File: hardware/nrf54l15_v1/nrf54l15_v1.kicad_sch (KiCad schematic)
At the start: 2 parts, among them U1 MAXM86161EFD+, U2 VL53L0X

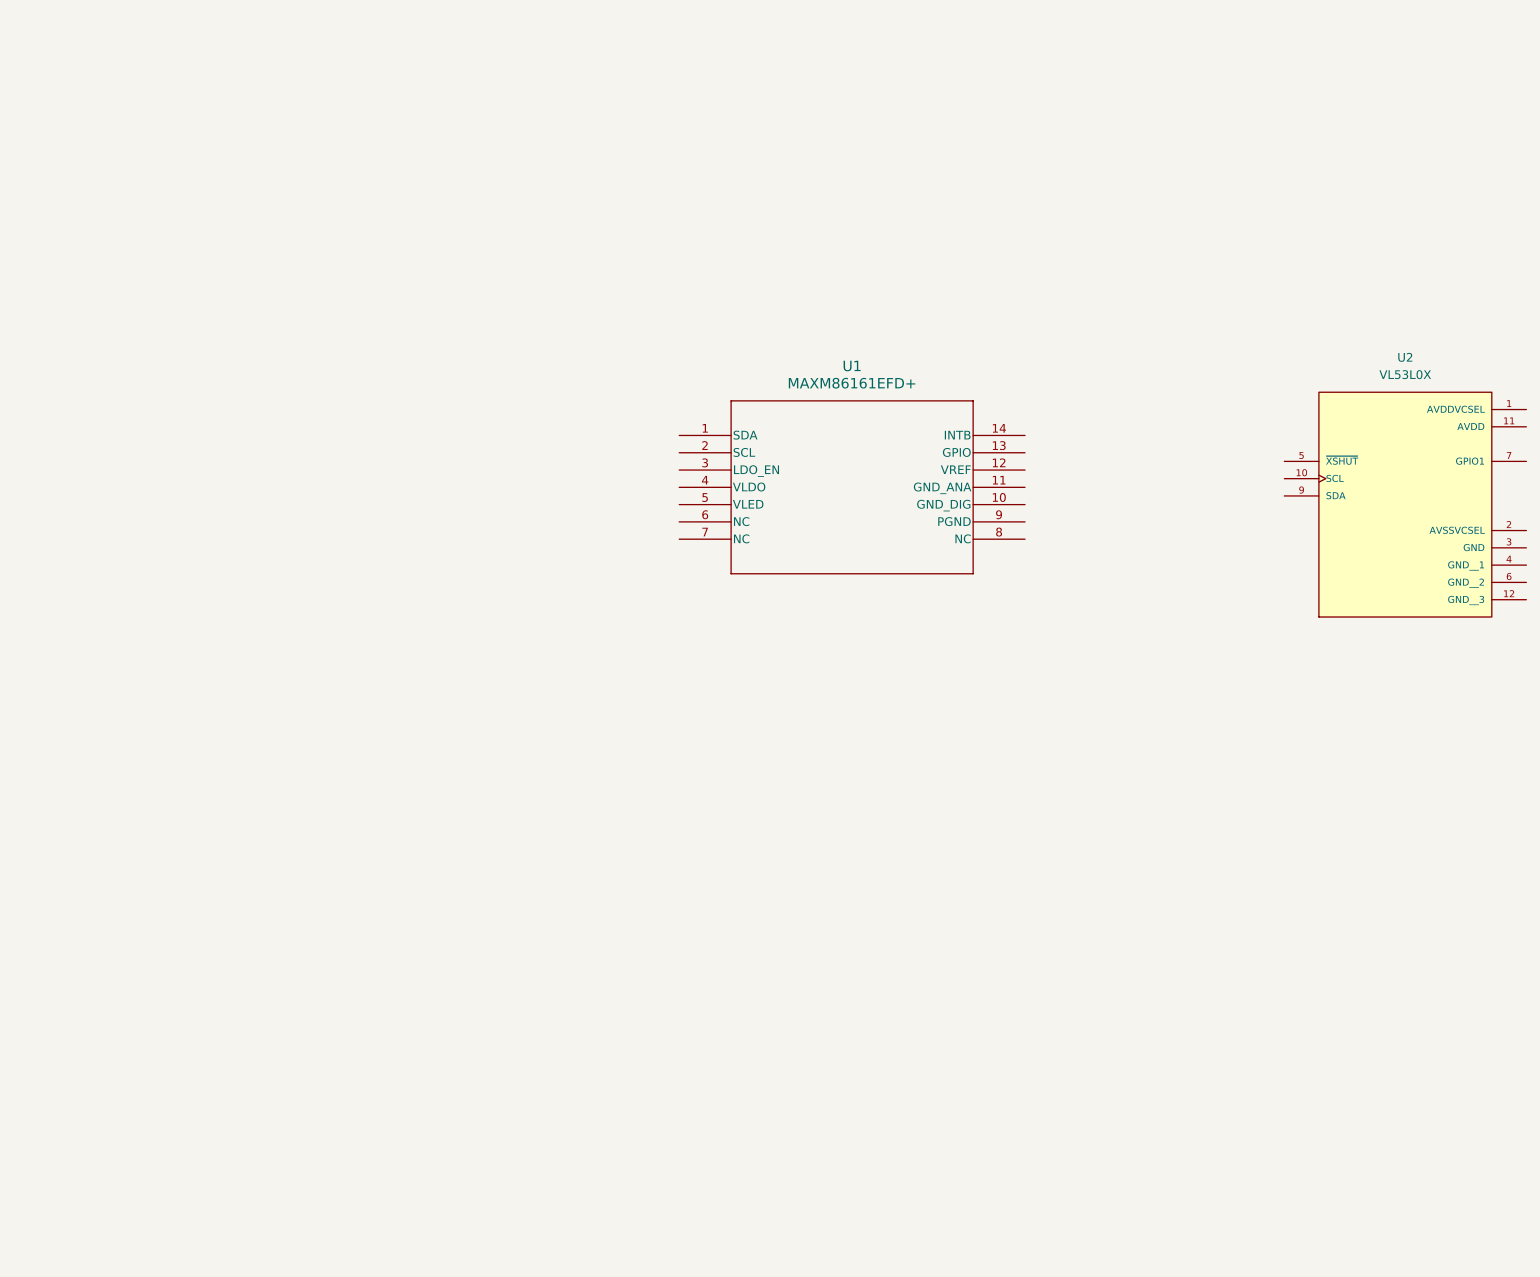
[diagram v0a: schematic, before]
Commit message: samples push
samples push
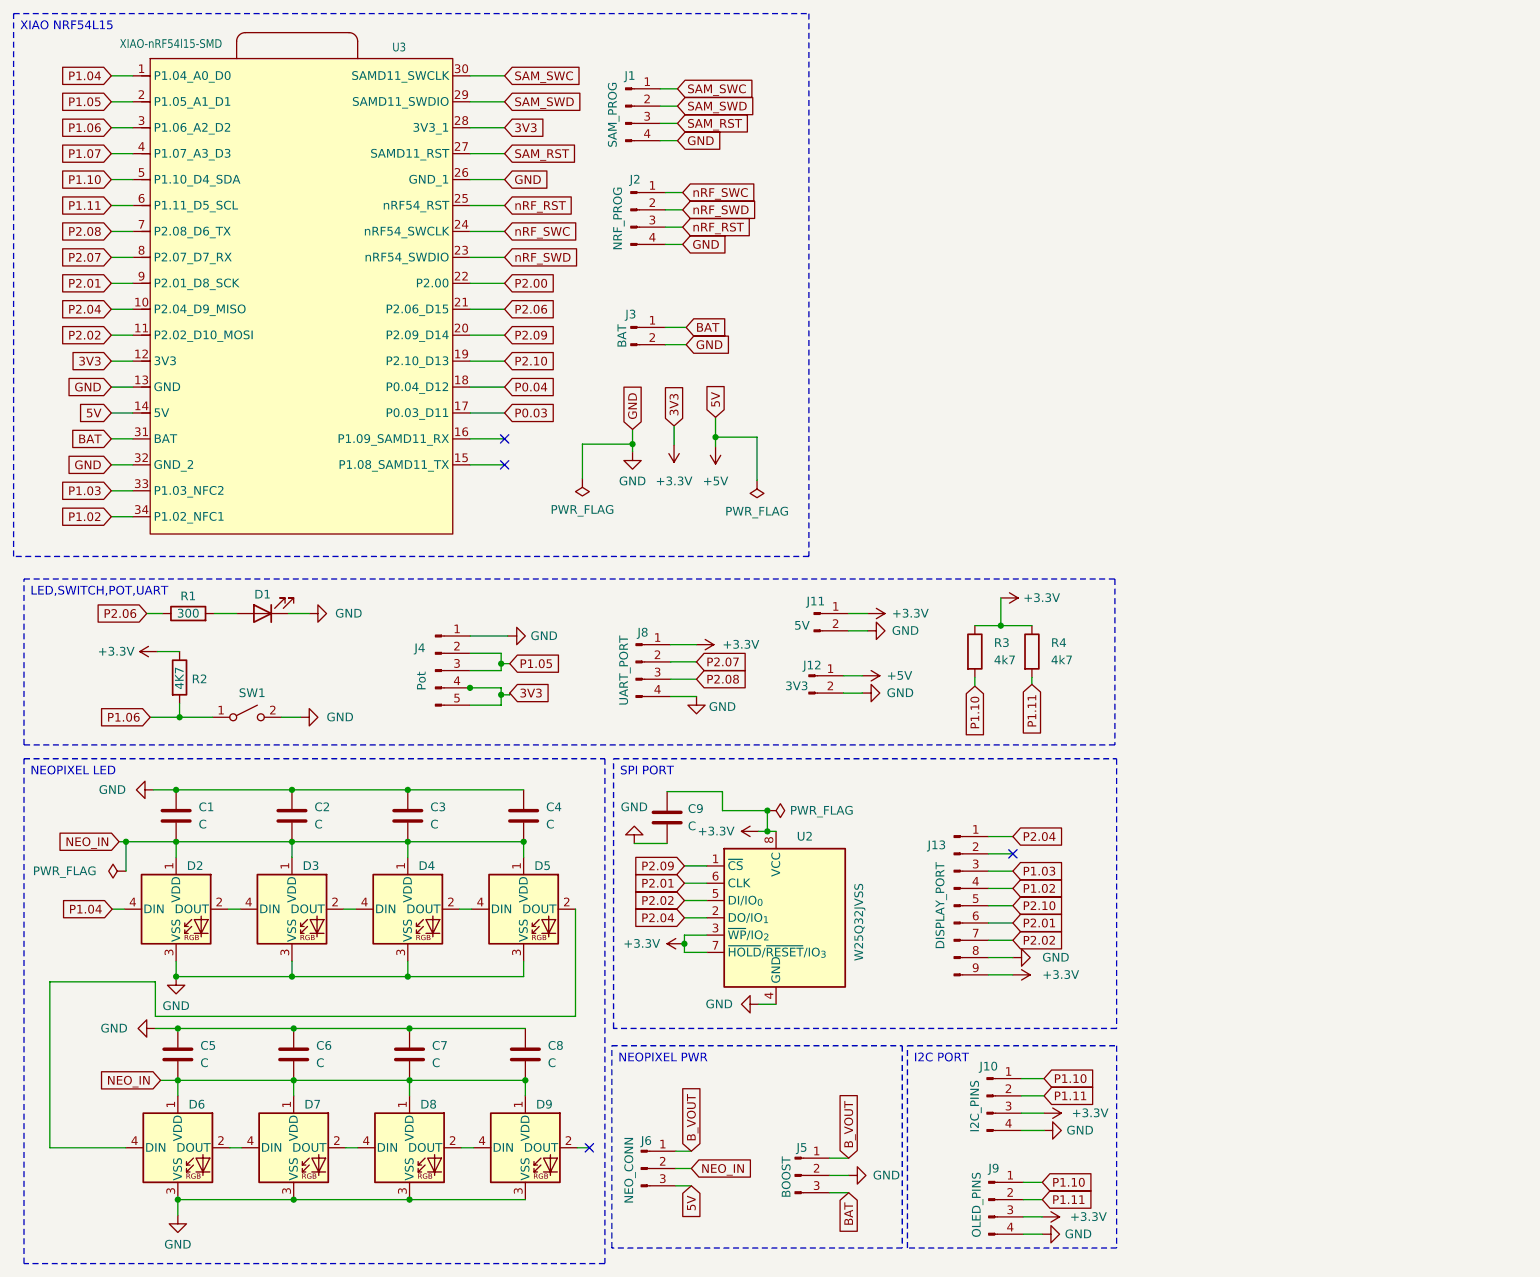
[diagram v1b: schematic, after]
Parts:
- removed U1: MAXM86161EFD+, 21-100309A_MXM, symbol maxm86161:MAXM86161EFD+
- removed U2: VL53L0X, VL53L0X:SENSOR_VL53L0X, symbol vl53l0x:VL53L0X
- added C1, C2, C3, C4, C5, C6, C7, C8, C9: C, Capacitor_SMD:C_0805_2012Metric_Pad1.18x1.45mm_HandSolder, symbol Device:C
- added D1: LED, LED_SMD:LED_0805_2012Metric_Pad1.15x1.40mm_HandSolder, symbol Device:LED
- added D2, D3, D4, D5, D6, D7, D8, D9: WS2812B, LED_SMD:LED_WS2812B_PLCC4_5.0x5.0mm_P3.2mm, symbol LED:WS2812B
- added J1: SAM_PROG, Connector_JST:JST_XH_S4B-XH-A_1x04_P2.50mm_Horizontal, symbol Connector:Conn_01x04_Pin
- added J10: I2C_PINS, Connector_JST:JST_XH_S4B-XH-A_1x04_P2.50mm_Horizontal, symbol Connector:Conn_01x04_Pin
- added J11: 5V, Connector_JST:JST_XH_S2B-XH-A-1_1x02_P2.50mm_Horizontal, symbol Connector:Conn_01x02_Pin
- added J12: 3V3, Connector_JST:JST_XH_S2B-XH-A-1_1x02_P2.50mm_Horizontal, symbol Connector:Conn_01x02_Pin
- added J13: DISPLAY_PORT, Connector_JST:JST_XH_S9B-XH-A-1_1x09_P2.50mm_Horizontal, symbol Connector:Conn_01x09_Pin
- added J2: NRF_PROG, Connector_JST:JST_XH_S4B-XH-A_1x04_P2.50mm_Horizontal, symbol Connector:Conn_01x04_Pin
- added J3: BAT, Connector_JST:JST_XH_S2B-XH-A-1_1x02_P2.50mm_Horizontal, symbol Connector:Conn_01x02_Pin
- added J4: Pot, Connector_PinSocket_2.54mm:PinSocket_1x05_P2.54mm_Vertical, symbol Connector:Conn_01x05_Pin
- added J5: BOOST, Connector_PinSocket_2.54mm:PinSocket_1x03_P2.54mm_Vertical, symbol Connector:Conn_01x03_Pin
- added J6: NEO_CONN, Connector_PinSocket_2.54mm:PinSocket_1x03_P2.54mm_Vertical, symbol Connector:Conn_01x03_Pin
- added J8: UART_PORT, Connector_JST:JST_XH_S4B-XH-A-1_1x04_P2.50mm_Horizontal, symbol Connector:Conn_01x04_Pin
- added J9: OLED_PINS, Connector_PinHeader_2.54mm:PinHeader_1x04_P2.54mm_Vertical, symbol Connector:Conn_01x04_Pin
- added R1: 300, Resistor_SMD:R_0805_2012Metric_Pad1.20x1.40mm_HandSolder, symbol Device:R
- added R2: 4K7, Resistor_SMD:R_0805_2012Metric_Pad1.20x1.40mm_HandSolder, symbol Device:R
- added R3, R4: 4k7, Resistor_SMD:R_0805_2012Metric_Pad1.20x1.40mm_HandSolder, symbol Device:R
- added SW1: SW_SPST, Button_Switch_SMD:SW_SPST_PTS647_Sx38, symbol Switch:SW_SPST
- added U2: W25Q32JVSS, Package_SO:SOIC-8_5.3x5.3mm_P1.27mm, symbol Memory_Flash:W25Q32JVSS
- added U3: XIAO-nRF54l15-SMD, xiao_nrf54l15:ym_, symbol YM_XIAO_nRF54:XIAO-nRF54l15-SMD
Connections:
- new net: D4.2 (DOUT), D5.4 (DIN)
- new net: D3.2 (DOUT), D4.4 (DIN)
- new net: D2.2 (DOUT), D3.4 (DIN)
- new net: D5.2 (DOUT), D6.4 (DIN)
- new net: D8.2 (DOUT), D9.4 (DIN)
- new net: D7.2 (DOUT), D8.4 (DIN)
- new net: D6.2 (DOUT), D7.4 (DIN)
- new net: D1.2 (A), R1.2
- new net +3.3V: C9.2, J10.3 (Pin_3), J11.1 (Pin_1), J13.9 (Pin_9), J4.4 (Pin_4), J4.5 (Pin_5), J8.1 (Pin_1), J9.3 (Pin_3), R2.1, R3.1, R4.1, U2.3 (~{WP}/IO_{2}), U2.7 (~{HOLD}/~{RESET}/IO_{3}), U2.8 (VCC), U3.12 (3V3), U3.28 (3V3_1)
- new net +5V: J12.1 (Pin_1), J6.3 (Pin_3), U3.14 (5V)
- new net BAT: J3.1 (Pin_1), J5.3 (Pin_3), U3.31 (BAT)
- new net B_VOUT: J5.1 (Pin_1), J6.1 (Pin_1)
- new net GND: C1.1, C2.1, C3.1, C4.1, C5.1, C6.1, C7.1, C8.1, C9.1, D1.1 (K), D2.3 (VSS), D3.3 (VSS), D4.3 (VSS), D5.3 (VSS), D6.3 (VSS), D7.3 (VSS), D8.3 (VSS), D9.3 (VSS), J1.4 (Pin_4), J10.4 (Pin_4), J11.2 (Pin_2), J12.2 (Pin_2), J13.8 (Pin_8), J2.4 (Pin_4), J3.2 (Pin_2), J4.1 (Pin_1), J5.2 (Pin_2), J8.4 (Pin_4), J9.4 (Pin_4), SW1.2 (B), U2.4 (GND), U3.13 (GND), U3.26 (GND_1), U3.32 (GND_2)
- new net NEO_IN: C1.2, C2.2, C3.2, C4.2, C5.2, C6.2, C7.2, C8.2, D2.1 (VDD), D3.1 (VDD), D4.1 (VDD), D5.1 (VDD), D6.1 (VDD), D7.1 (VDD), D8.1 (VDD), D9.1 (VDD), J6.2 (Pin_2)
- new net P0.03: U3.17 (P0.03_D11)
- new net P0.04: U3.18 (P0.04_D12)
- new net P1.02: J13.4 (Pin_4), U3.34 (P1.02_NFC1)
- new net P1.03: J13.3 (Pin_3), U3.33 (P1.03_NFC2)
- new net P1.04: D2.4 (DIN), U3.1 (P1.04_A0_D0)
- new net P1.05: J4.2 (Pin_2), J4.3 (Pin_3), U3.2 (P1.05_A1_D1)
- new net P1.06: R2.2, SW1.1 (A), U3.3 (P1.06_A2_D2)
- new net P1.07: U3.4 (P1.07_A3_D3)
- new net P1.10: J10.1 (Pin_1), J9.1 (Pin_1), R3.2, U3.5 (P1.10_D4_SDA)
- new net P1.11: J10.2 (Pin_2), J9.2 (Pin_2), R4.2, U3.6 (P1.11_D5_SCL)
- new net P2.00: U3.22 (P2.00)
- new net P2.01: J13.6 (Pin_6), U2.6 (CLK), U3.9 (P2.01_D8_SCK)
- new net P2.02: J13.7 (Pin_7), U2.5 (DI/IO_{0}), U3.11 (P2.02_D10_MOSI)
- new net P2.04: J13.1 (Pin_1), U2.2 (DO/IO_{1}), U3.10 (P2.04_D9_MISO)
- new net P2.06: R1.1, U3.21 (P2.06_D15)
- new net P2.07: J8.2 (Pin_2), U3.8 (P2.07_D7_RX)
- new net P2.08: J8.3 (Pin_3), U3.7 (P2.08_D6_TX)
- new net P2.09: U2.1 (~{CS}), U3.20 (P2.09_D14)
- new net P2.10: J13.5 (Pin_5), U3.19 (P2.10_D13)
- new net SAM_RST: J1.3 (Pin_3), U3.27 (SAMD11_RST)
- new net SAM_SWC: J1.1 (Pin_1), U3.30 (SAMD11_SWCLK)
- new net SAM_SWD: J1.2 (Pin_2), U3.29 (SAMD11_SWDIO)
- new net nRF_RST: J2.3 (Pin_3), U3.25 (nRF54_RST)
- new net nRF_SWC: J2.1 (Pin_1), U3.24 (nRF54_SWCLK)
- new net nRF_SWD: J2.2 (Pin_2), U3.23 (nRF54_SWDIO)
- no-connect marks 0 -> 4
